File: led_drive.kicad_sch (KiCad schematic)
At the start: 0 parts

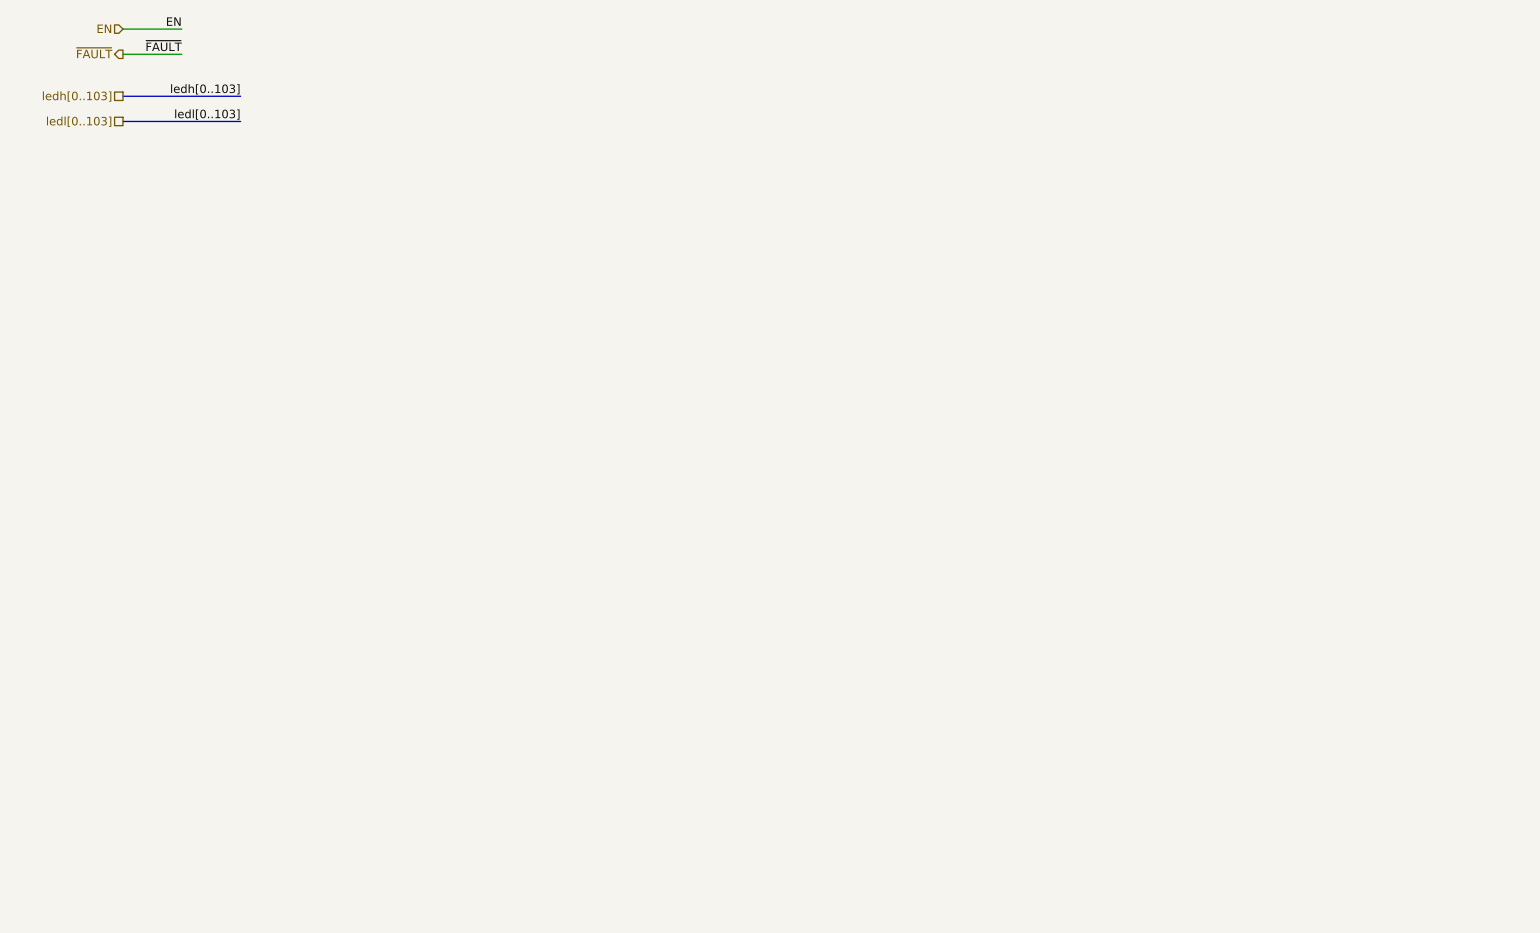
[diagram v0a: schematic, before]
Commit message: Fleshed out layout
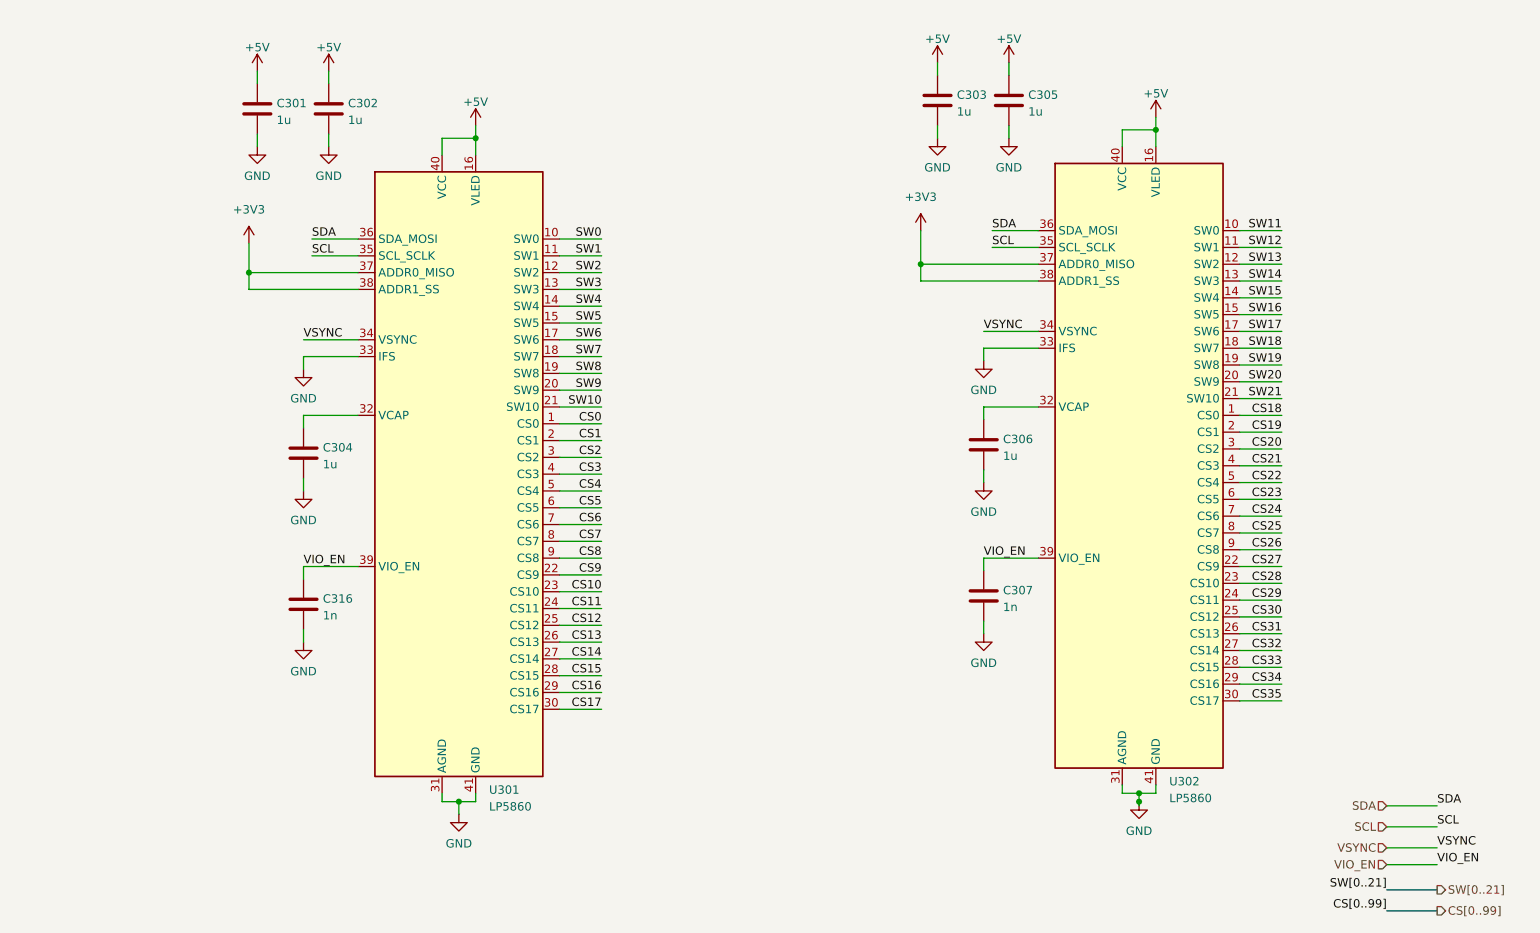
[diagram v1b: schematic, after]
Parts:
- added C301, C302, C303, C304, C305, C306: 1u, Capacitor_SMD:C_0603_1608Metric, symbol Device:C
- added C307, C316: 1n, Capacitor_SMD:C_0603_1608Metric, symbol Device:C
- added U301, U302: LP5860, Package_DFN_QFN:QFN-40-1EP_5x5mm_P0.4mm_EP3.8x3.8mm_ThermalVias, symbol Keyboard:LP5860
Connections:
- new net: C304.1, U301.32 (VCAP)
- new net: C306.1, U302.32 (VCAP)
- new net +3V3: U301.37 (ADDR0_MISO), U301.38 (ADDR1_SS), U302.37 (ADDR0_MISO), U302.38 (ADDR1_SS)
- new net +5V: C301.1, C302.1, C303.1, C305.1, U301.16 (VLED), U301.40 (VCC), U302.16 (VLED), U302.40 (VCC)
- new net CS0: U301.1 (CS0)
- new net CS1: U301.2 (CS1)
- new net CS10: U301.23 (CS10)
- new net CS11: U301.24 (CS11)
- new net CS12: U301.25 (CS12)
- new net CS13: U301.26 (CS13)
- new net CS14: U301.27 (CS14)
- new net CS15: U301.28 (CS15)
- new net CS16: U301.29 (CS16)
- new net CS17: U301.30 (CS17)
- new net CS18: U302.1 (CS0)
- new net CS19: U302.2 (CS1)
- new net CS2: U301.3 (CS2)
- new net CS20: U302.3 (CS2)
- new net CS21: U302.4 (CS3)
- new net CS22: U302.5 (CS4)
- new net CS23: U302.6 (CS5)
- new net CS24: U302.7 (CS6)
- new net CS25: U302.8 (CS7)
- new net CS26: U302.9 (CS8)
- new net CS27: U302.22 (CS9)
- new net CS28: U302.23 (CS10)
- new net CS29: U302.24 (CS11)
- new net CS3: U301.4 (CS3)
- new net CS30: U302.25 (CS12)
- new net CS31: U302.26 (CS13)
- new net CS32: U302.27 (CS14)
- new net CS33: U302.28 (CS15)
- new net CS34: U302.29 (CS16)
- new net CS35: U302.30 (CS17)
- new net CS4: U301.5 (CS4)
- new net CS5: U301.6 (CS5)
- new net CS6: U301.7 (CS6)
- new net CS7: U301.8 (CS7)
- new net CS8: U301.9 (CS8)
- new net CS9: U301.22 (CS9)
- new net GND: C301.2, C302.2, C303.2, C304.2, C305.2, C306.2, C307.2, C316.2, U301.31 (AGND), U301.33 (IFS), U301.41 (GND), U302.31 (AGND), U302.33 (IFS), U302.41 (GND)
- new net SCL: U301.35 (SCL_SCLK), U302.35 (SCL_SCLK)
- new net SDA: U301.36 (SDA_MOSI), U302.36 (SDA_MOSI)
- new net SW0: U301.10 (SW0)
- new net SW1: U301.11 (SW1)
- new net SW10: U301.21 (SW10)
- new net SW11: U302.10 (SW0)
- new net SW12: U302.11 (SW1)
- new net SW13: U302.12 (SW2)
- new net SW14: U302.13 (SW3)
- new net SW15: U302.14 (SW4)
- new net SW16: U302.15 (SW5)
- new net SW17: U302.17 (SW6)
- new net SW18: U302.18 (SW7)
- new net SW19: U302.19 (SW8)
- new net SW2: U301.12 (SW2)
- new net SW20: U302.20 (SW9)
- new net SW21: U302.21 (SW10)
- new net SW3: U301.13 (SW3)
- new net SW4: U301.14 (SW4)
- new net SW5: U301.15 (SW5)
- new net SW6: U301.17 (SW6)
- new net SW7: U301.18 (SW7)
- new net SW8: U301.19 (SW8)
- new net SW9: U301.20 (SW9)
- new net VIO_EN: C307.1, C316.1, U301.39 (VIO_EN), U302.39 (VIO_EN)
- new net VSYNC: U301.34 (VSYNC), U302.34 (VSYNC)
